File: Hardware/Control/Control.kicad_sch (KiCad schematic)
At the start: 44 parts, among them SW1 EN11-HSM1AF20, SW2 KO128B2007, SW3 Conn_01x04, U1 XRA1402IG16TR-F, U2 FT230XS-U, U4 ATMEGA328P-AU, U5 ESDALD05UD4, Y1 ABM8AIG-20.000MHZ-4-T

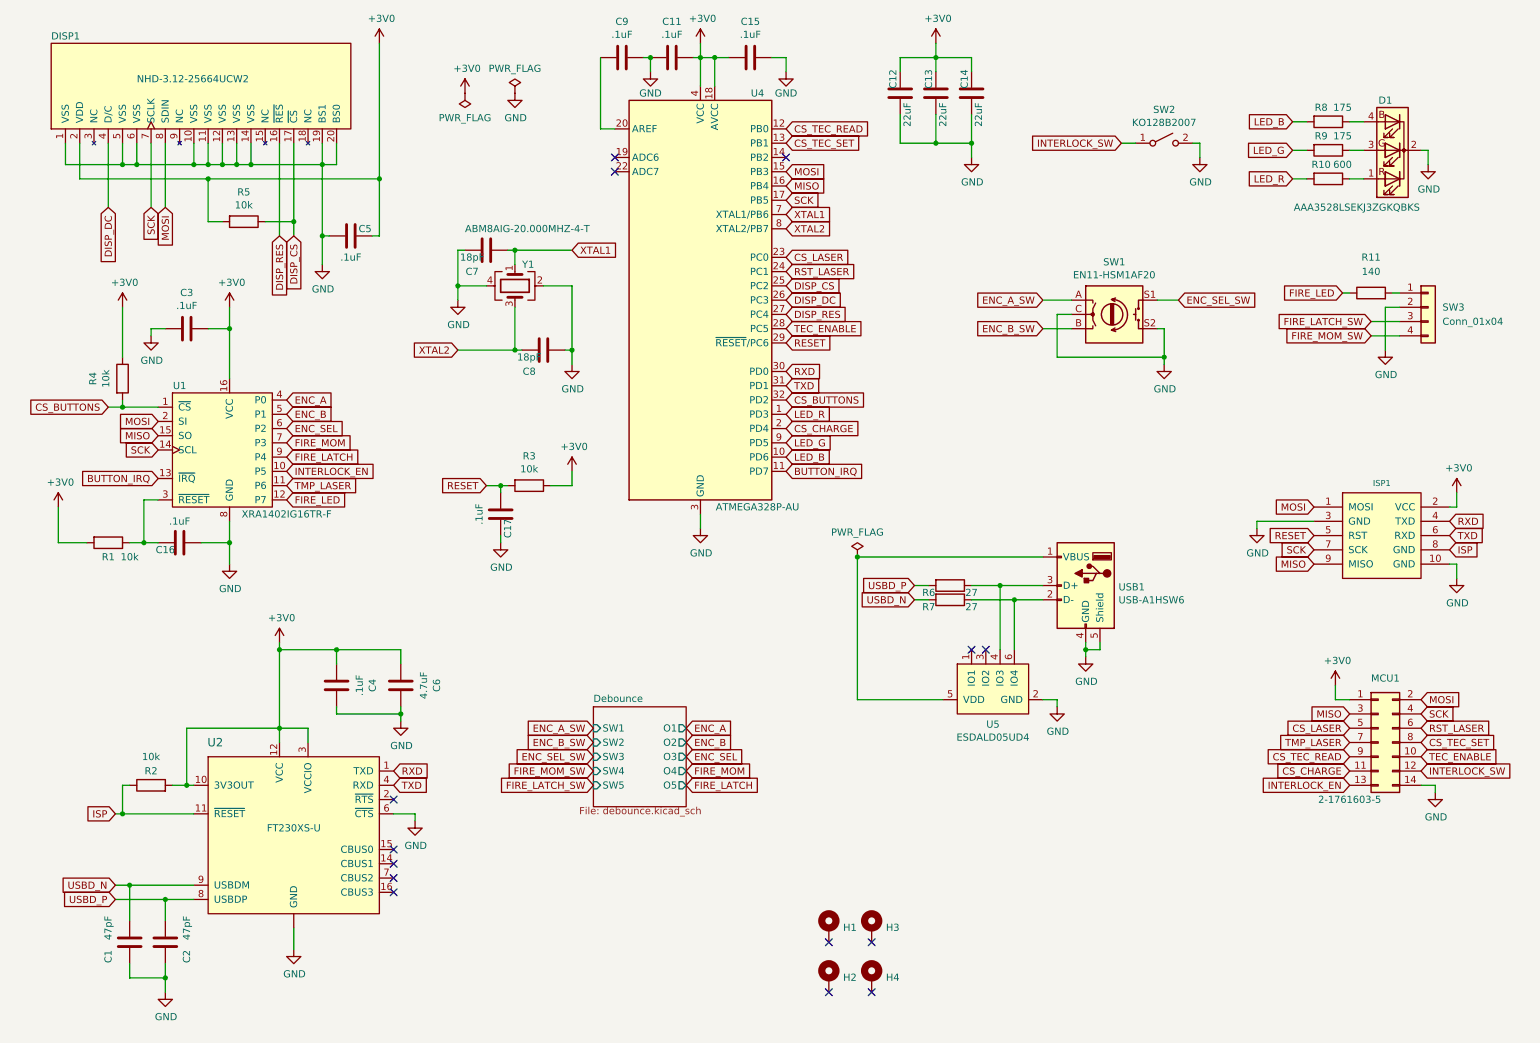
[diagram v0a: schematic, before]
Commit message: Merge revision 2.1 into main
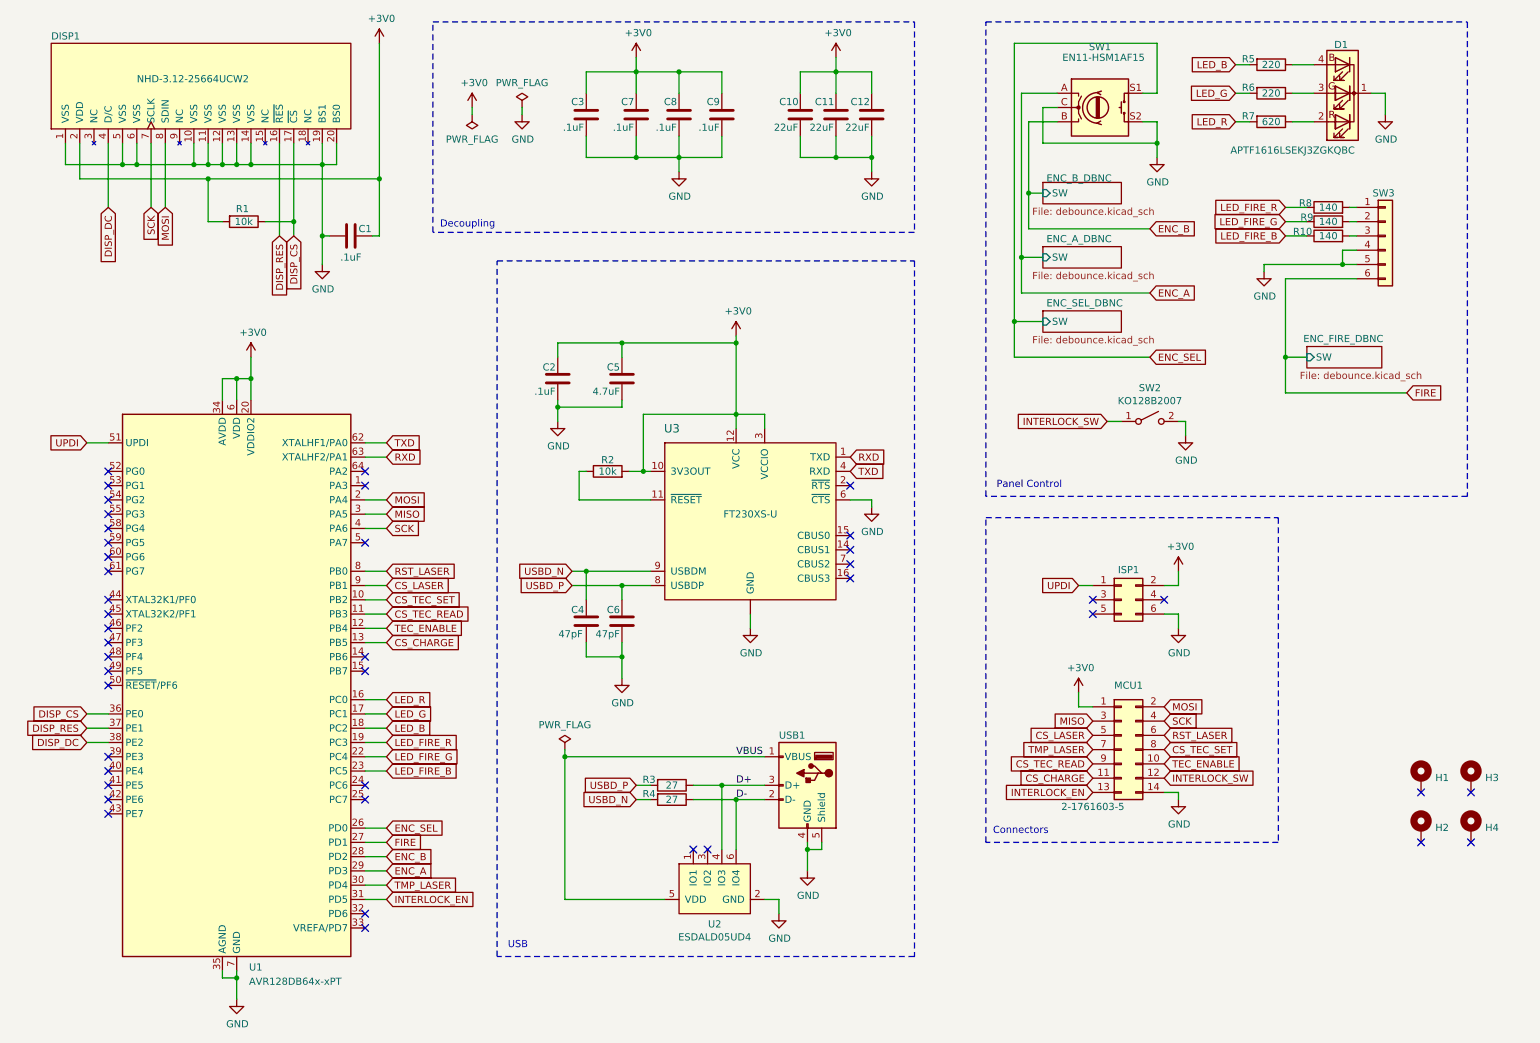
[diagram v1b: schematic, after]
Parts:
- removed C11, C15, C16, C17: .1uF, Capacitor_SMD:C_0805_2012Metric, symbol Device:C
- removed D1: AAA3528LSEKJ3ZGKQBKS, LED_SMD:LED_Avago_PLCC4_3.2x2.8mm_CW, symbol Device:LED_RKGB
- removed ISP1: AVR_ISP_10_SERIAL, pepin-footprints:TC2050-IDC, symbol pepin_con:AVR_ISP_10_SERIAL
- removed R1, R3, R4: 10k, Resistor_SMD:R_0805_2012Metric, symbol Device:R
- removed SW3: Conn_01x04, Connector_PinHeader_2.54mm:PinHeader_1x04_P2.54mm_Vertical, symbol Connector_Generic:Conn_01x04
- removed U1: XRA1402IG16TR-F, Package_SO:TSSOP-16_4.4x5mm_P0.65mm, symbol Components:XRA1402IG16TR-F
- removed U4: ATMEGA328P-AU, Package_QFP:TQFP-32_7x7mm_P0.8mm, symbol MCU_Microchip_ATmega:ATmega328P-A
- removed Y1: ABM8AIG-20.000MHZ-4-T, Crystal:Crystal_SMD_3225-4Pin_3.2x2.5mm, symbol Device:Crystal_GND24
- added D1: APTF1616LSEKJ3ZGKQBC, Components:LED_Kingbright_KRGB_1.6x1.6mm, symbol Device:LED_KRGB
- added ISP1: 61200621621, Connector_IDC:IDC-Header_2x03_P2.54mm_Vertical, symbol Connector_Generic:Conn_02x03_Odd_Even
- added R10, R9: 140, Resistor_SMD:R_0805_2012Metric, symbol Device:R
- added SW3: Conn_01x06, Connector_PinHeader_2.54mm:PinHeader_1x06_P2.54mm_Vertical, symbol Connector_Generic:Conn_01x06
- added U1: AVR128DB64x-xPT, Package_QFP:TQFP-64_10x10mm_P0.5mm, symbol MCU_Microchip_AVR_Dx:AVR128DB64x-xPT
- C1: renamed from C5; Product Number (none) -> CGA4J2X8R1H104K125AE
- C10: renamed from C12; Product Number CL31A226KAHNNNE -> LMJ316BB7226KLHT
- C11: renamed from C13; Product Number CL31A226KAHNNNE -> LMJ316BB7226KLHT
- C12: renamed from C14; Product Number CL31A226KAHNNNE -> LMJ316BB7226KLHT
- C2: renamed from C4; Product Number (none) -> CGA4J2X8R1H104K125AE
- C3, C9: Product Number (none) -> CGA4J2X8R1H104K125AE
- C4: renamed from C1; Product Number (none) -> C0805C470J1GAC
- C5: renamed from C6; Product Number (none) -> C0805C475K4RACAUTO
- C6: renamed from C2; Product Number (none) -> C0805C470J1GAC
- C7, C8: value 18pF -> .1uF; Product Number C0805C180J5HACTU -> CGA4J2X8R1H104K125AE
- R1: renamed from R5; Product Number (none) -> ERA-6AEB103V
- R2: Product Number (none) -> ERA-6AEB103V
- R3: renamed from R6; Product Number (none) -> CR0805-FX-27R0ELF
- R4: renamed from R7; Product Number (none) -> CR0805-FX-27R0ELF
- R5: renamed from R8; value 175 -> 220; Product Number (none) -> ERA-6AEB221V
- R6: renamed from R9; value 175 -> 220; Product Number (none) -> ERA-6AEB221V
- R7: renamed from R10; value 600 -> 620; Product Number (none) -> CR0805-FX-6200ELF
- R8: renamed from R11; Product Number (none) -> CRCW0805140RFKEA
- SW1: value EN11-HSM1AF20 -> EN11-HSM1AF15; Product Number EN11-HSM1AF20 -> EN11-HSM1AF15
- USB1: value USB-A1HSW6 -> UJ2-A-HR-G-TH; Product Number USB-A1HSW6 -> UJ2-A-HR-G-TH
- renumbered U5 to U2, U2 to U3
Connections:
- net ENC_A_SW is gone; now on net ENC_A: SW1.A
- net ENC_B_SW is gone; now on net ENC_B: SW1.B
- net ENC_SEL_SW is gone; now on net ENC_SEL: SW1.S1
- net XTAL1 is gone; now on net GND: C7.1
- net XTAL2 is gone; now on net +3V0: C8.2
- net +3V0: now also C7.2, C9.2, ISP1.2 (Pin_2), U1.20 (VDDIO2), U1.34 (AVDD), U1.56 (VDD), U1.6 (VDD)
- net CS_CHARGE: now also U1.13 (PB5)
- net CS_LASER: now also U1.9 (PB1)
- net CS_TEC_READ: now also U1.11 (PB3)
- net CS_TEC_SET: now also U1.10 (PB2)
- net DISP_CS: now also U1.36 (PE0)
- net DISP_DC: now also U1.38 (PE2)
- net DISP_RES: now also U1.37 (PE1)
- net ENC_A: now also U1.29 (PD3)
- net ENC_B: now also U1.28 (PD2)
- net ENC_SEL: now also U1.26 (PD0)
- net GND: now also C9.1, D1.1 (K), ISP1.6 (Pin_6), SW3.4 (Pin_4), SW3.5 (Pin_5), U1.21 (GND), U1.35 (AGND), U1.57 (GND), U1.7 (GND); no longer C7.2, C9.2
- net INTERLOCK_EN: now also U1.31 (PD5)
- net LED_B: now also U1.18 (PC2)
- net LED_G: now also U1.17 (PC1)
- net LED_R: now also U1.16 (PC0)
- net MISO: now also U1.3 (PA5)
- net MOSI: now also U1.2 (PA4)
- net RST_LASER: now also U1.8 (PB0)
- net RXD: now also U1.63 (XTALHF2/PA1)
- net SCK: now also U1.4 (PA6)
- net TEC_ENABLE: now also U1.12 (PB4)
- net TMP_LASER: now also U1.30 (PD4)
- net TXD: now also U1.62 (XTALHF1/PA0)
- net at R5.1: now also D1.4 (BA)
- net at R6.1: now also D1.3 (GA)
- net at R7.1: now also D1.2 (RA)
- net VBUS: now reaches U2.5 (VDD), USB1.1 (VBUS)
- net D-: now reaches R4.1, U2.6 (IO4), USB1.2 (D-)
- net D+: now reaches R3.1, U2.4 (IO3), USB1.3 (D+)
- net at R8.2: now also SW3.1 (Pin_1)
- net FIRE_LED renamed LED_FIRE_R
- net LED_FIRE_R: now also U1.19 (PC3)
- net ISP: no longer names the net of R2.1, U3.11 (~{RESET})
- new net: R9.2, SW3.2 (Pin_2)
- new net: R10.2, SW3.3 (Pin_3)
- new net FIRE: SW3.6 (Pin_6), U1.27 (PD1)
- new net LED_FIRE_B: R10.1, U1.23 (PC5)
- new net LED_FIRE_G: R9.1, U1.22 (PC4)
- new net UPDI: ISP1.1 (Pin_1), U1.51 (UPDI)
- no-connect marks 14 -> 43
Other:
- removed sheet Debounce
- added sheet ENC_A_DBNC (debounce.kicad_sch)
- added sheet ENC_B_DBNC (debounce.kicad_sch)
- added sheet ENC_FIRE_DBNC (debounce.kicad_sch)
- added sheet ENC_SEL_DBNC (debounce.kicad_sch)
- note added: "Connectors"
- note added: "Decoupling"
- note added: "Panel Control"
- note added: "USB"
- moved on the sheet: C10, C11, C12, C2, C4, C5, C6, H1, H2, H3, H4, MCU1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
